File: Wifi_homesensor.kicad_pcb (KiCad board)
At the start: 2 copper layers, 53.3 x 64.4 mm, 20 parts, among them J1 Pinhdr 3x2.5, U1 MCP16301, U2 WeMos_D1_mini, U3 SHT31-DIS

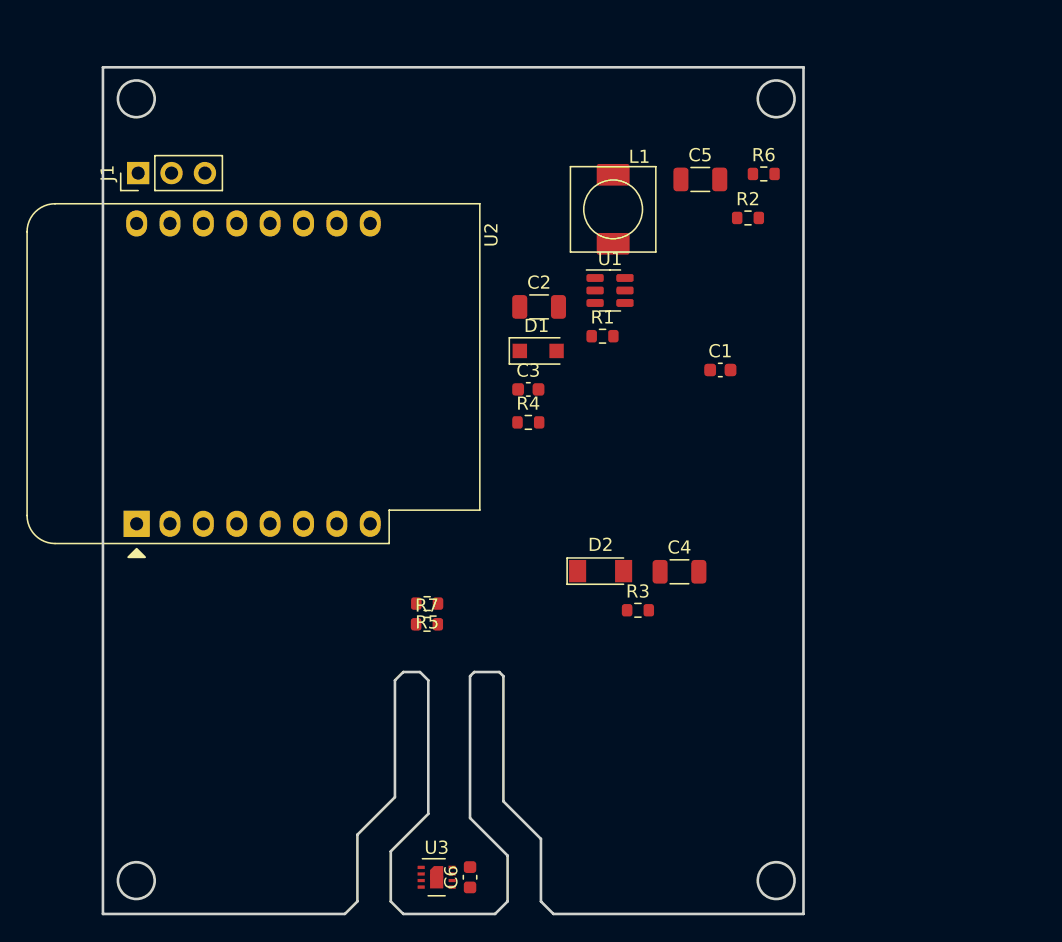
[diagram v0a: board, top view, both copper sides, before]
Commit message: schematic finished, pcb editing started
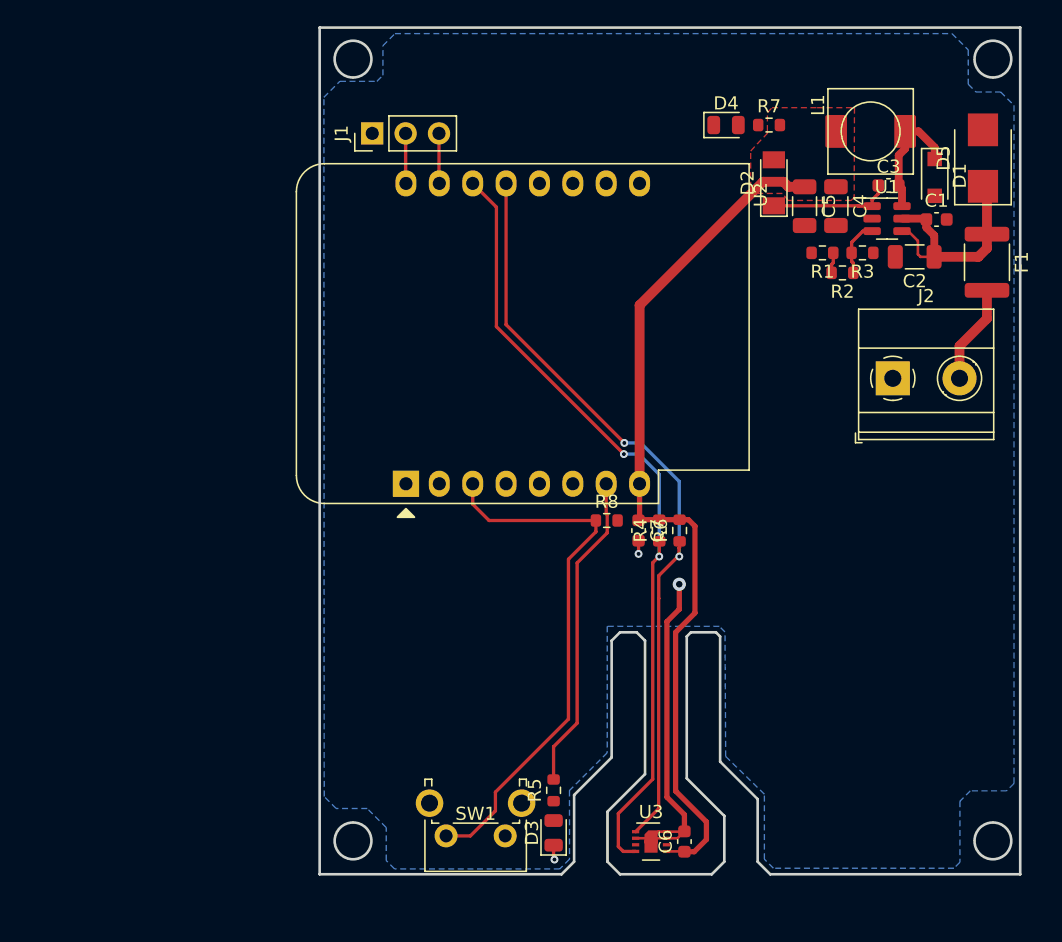
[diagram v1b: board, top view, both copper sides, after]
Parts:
- added C7: 100nF, Capacitor_SMD:C_0603_1608Metric, F.Cu at (144.8, 103.4)
- added D3: LED, LED_SMD:LED_0805_2012Metric, F.Cu at (138.3, 126.4)
- added D4: LED, LED_SMD:LED_0805_2012Metric, F.Cu at (151.4, 72.5)
- added D5: SM6T15A, Diode_SMD:D_SMB, F.Cu at (171.0, 75.1)
- added F1: 100mA, Fuse:Fuse_1812_4532Metric, F.Cu at (171.3, 83.0)
- added J2: Conn_01x02, TerminalBlock_Phoenix:TerminalBlock_Phoenix_MKDS-1,5-2-5.08_1x02_P5.08mm_Horizontal, F.Cu at (164.1, 91.8)
- added R8: 10k, Resistor_SMD:R_0603_1608Metric, F.Cu at (142.4, 102.6)
- added SW1: SW_Push, Button_Switch_THT:SW_Tactile_SPST_Angled_PTS645Vx83-2LFS, F.Cu at (134.6, 126.6)
- moved R7 46.1 mm to (154.7, 72.5)
- moved D1 32.9 mm to (167.3, 76.5), turned to -90 degrees
- moved D2 32.4 mm to (155.1, 76.9), turned to 90 degrees
- moved R3 32.1 mm to (161.8, 82.3), turned to 180 degrees
- moved C3 31.5 mm to (163.8, 77.1)
- moved C4 30.3 mm to (159.8, 78.7), turned to -90 degrees
- moved C2 28.8 mm to (165.8, 82.6), turned to 180 degrees
- moved R6 27.9 mm to (147.9, 103.4), turned to 90 degrees
- moved U1 21.8 mm to (163.7, 79.7)
- moved U2 20.7 mm to (127.1, 99.8)
- moved L1 20.5 mm to (162.4, 73.0), turned to 90 degrees
- moved C1 20.1 mm to (167.5, 79.7)
- moved J1 18.1 mm to (124.5, 73.2)
- moved R1 17.9 mm to (158.8, 82.3), turned to 180 degrees
- moved R5 17.2 mm to (138.3, 123.2), turned to 90 degrees
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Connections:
- U2 pad 3: unconnected-(U2-Pad3) -> /CONFIG
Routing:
- net +3V3: track 0.00 -> 66.4 mm
- net /SCL: track 0.00 -> 61.0 mm, vias 0 -> 2
- net /SDA: track 0.00 -> 58.2 mm, vias 0 -> 2
- net /CONFIG: track 0.00 -> 41.3 mm
- net GND: track 0.00 -> 29.0 mm, vias 0 -> 3
- net Net-(R5-Pad2): track 0.00 -> 24.2 mm
- net +12V: track 0.00 -> 18.0 mm
- net Net-(C3-Pad2): track 0.00 -> 9.64 mm
- net Net-(C3-Pad1): track 0.00 -> 9.26 mm
- net Net-(J2-Pad2): track 0.00 -> 7.56 mm
- net Net-(R2-Pad1): track 0.00 -> 4.29 mm
- net Net-(J1-Pad2): track 0.00 -> 3.82 mm
- net Net-(J1-Pad3): track 0.00 -> 3.82 mm
- net Net-(R1-Pad1): track 0.00 -> 1.58 mm
- added copper zone on F.Cu, net +3V3
- added copper zone on B.Cu, net GND
